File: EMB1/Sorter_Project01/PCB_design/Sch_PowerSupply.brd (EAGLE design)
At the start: 100.1 x 81.2 mm, 13 parts, among them IC1 LM2574N-3.3, IC2 7812T, IC3 7806T

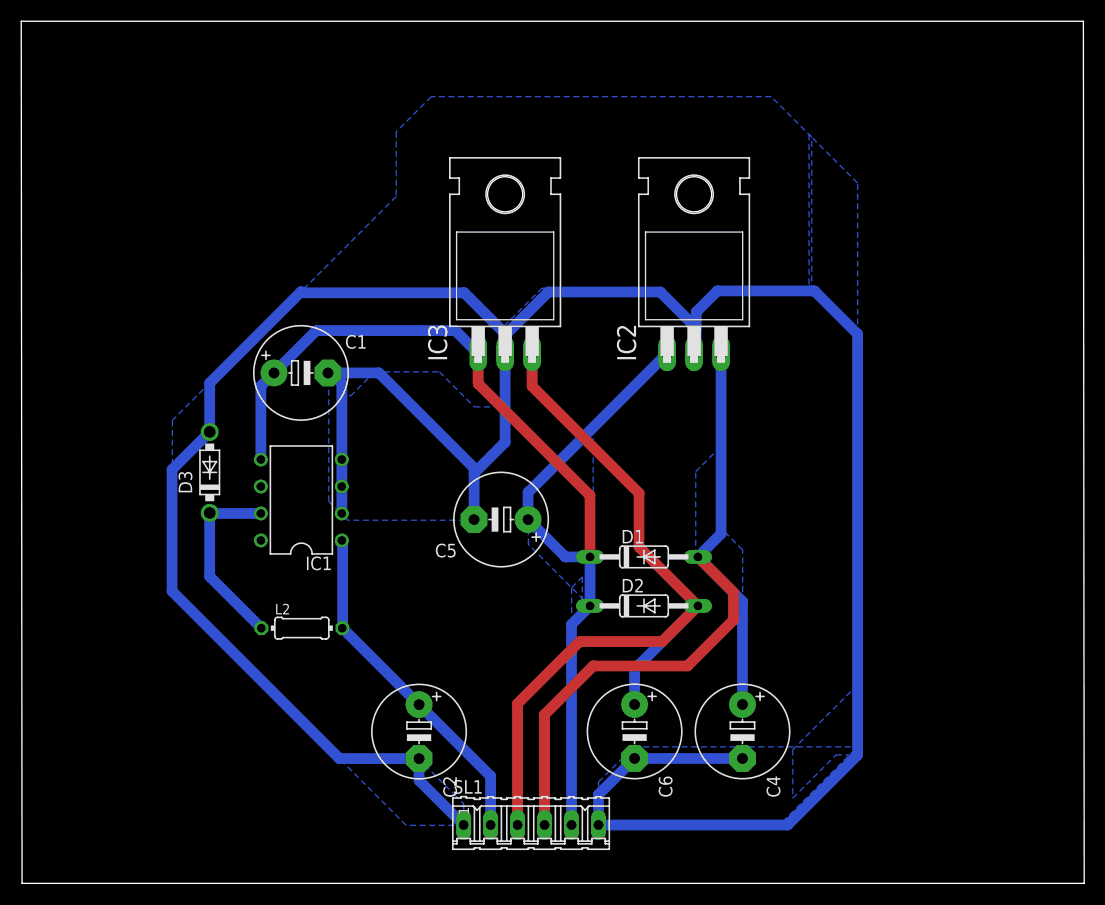
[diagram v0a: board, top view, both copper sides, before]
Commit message: New board
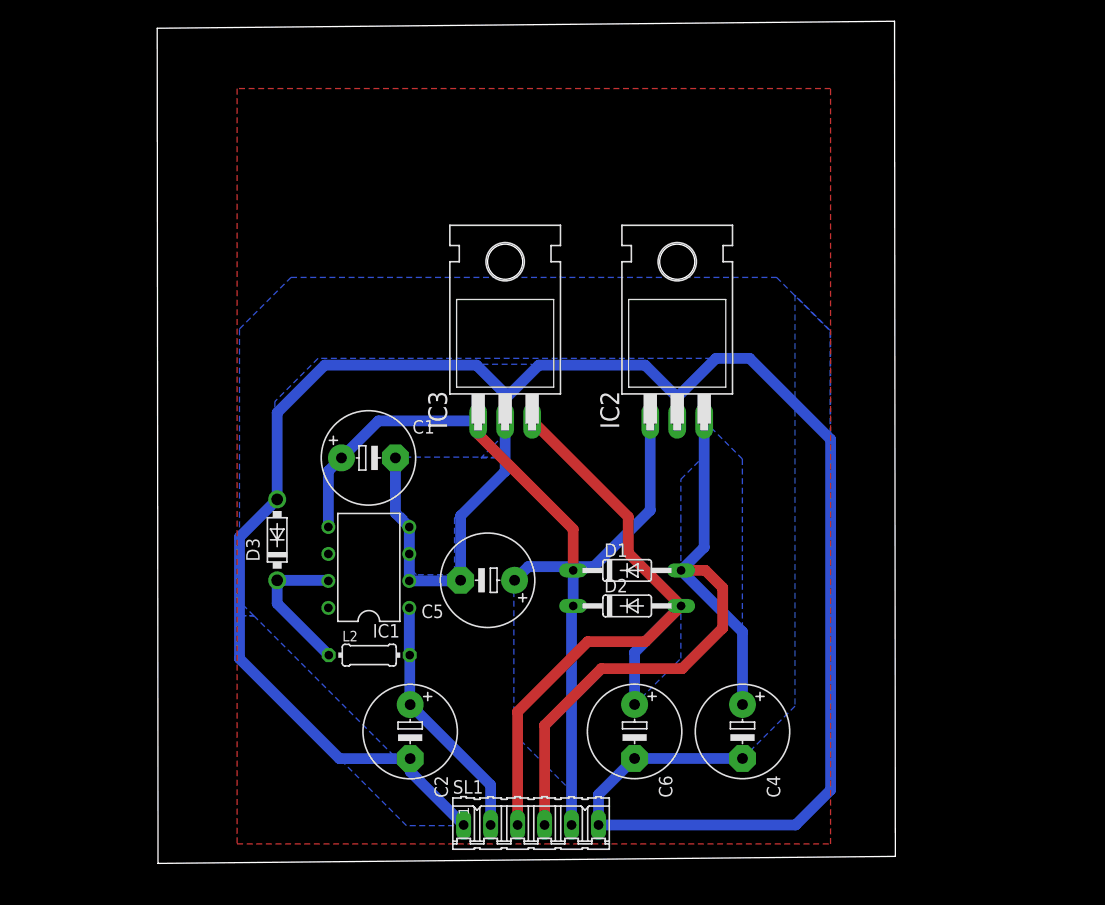
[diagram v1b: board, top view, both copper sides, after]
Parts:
- moved C1 10.2 mm to (32.7, 38.9)
- moved D3 8.98 mm to (24.1, 31.2)
- moved IC1 8.98 mm to (32.7, 28.6)
- moved L2 6.84 mm to (32.8, 20.3)
- moved IC2 6.55 mm to (61.8, 52.5)
- moved IC3 6.35 mm to (45.6, 52.5)
- moved C5 5.85 mm to (43.9, 27.4)
- moved D1 2.03 mm to (57.0, 28.3)
- moved D2 1.59 mm to (57.0, 25.0)
- moved C2 0.84 mm to (36.6, 13.1)
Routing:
- net GND: track 269.9 -> 227.8 mm
- net 15V: track 108.3 -> 89.0 mm
- net 6V: track 74.2 -> 64.5 mm
- net 5V: track 32.8 -> 23.6 mm
- net 12V: track 74.9 -> 68.3 mm
- net N$1: track 17.7 -> 13.9 mm
- added copper zone on layer 16, net 6V
- added copper zone on layer 1, net GND
- removed copper zone on layer 16, net 15V
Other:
- board size 100.1 x 81.2 mm -> 69.5 x 79.3 mm
